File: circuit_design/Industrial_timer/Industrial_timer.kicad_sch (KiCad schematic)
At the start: 31 parts, among them Q101 MMBT3904, Q103 DMP4065SQ, U101 SL78M05, U102 LM358_SIM

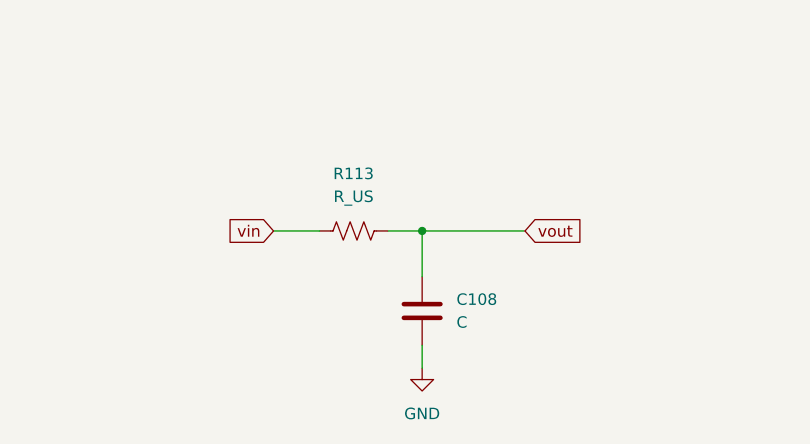
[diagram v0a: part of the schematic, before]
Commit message: Saving updated circuits.
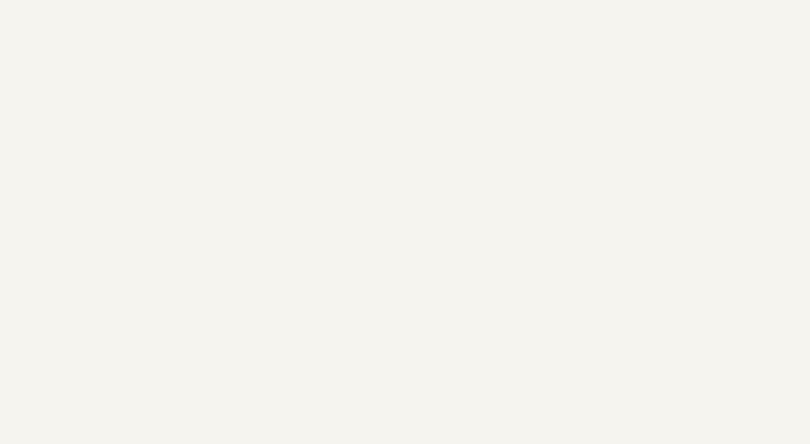
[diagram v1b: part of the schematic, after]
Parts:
- removed C108: C, symbol Device:C
- removed R113: R_US, symbol Device:R_US
